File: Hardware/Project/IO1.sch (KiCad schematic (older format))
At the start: 1 part, among them U8 8255

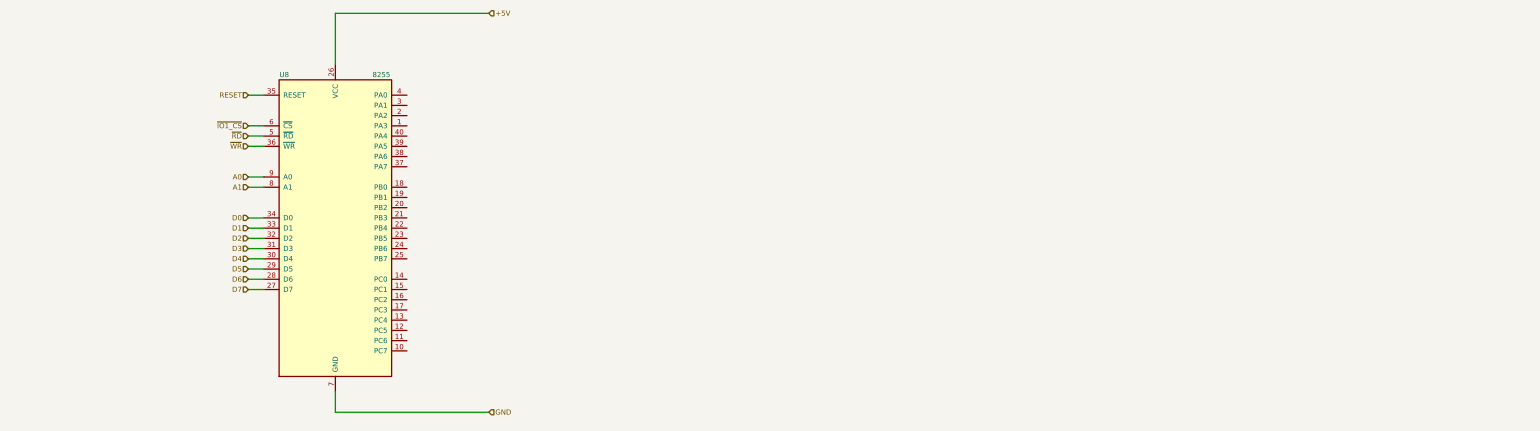
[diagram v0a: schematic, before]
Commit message: 1
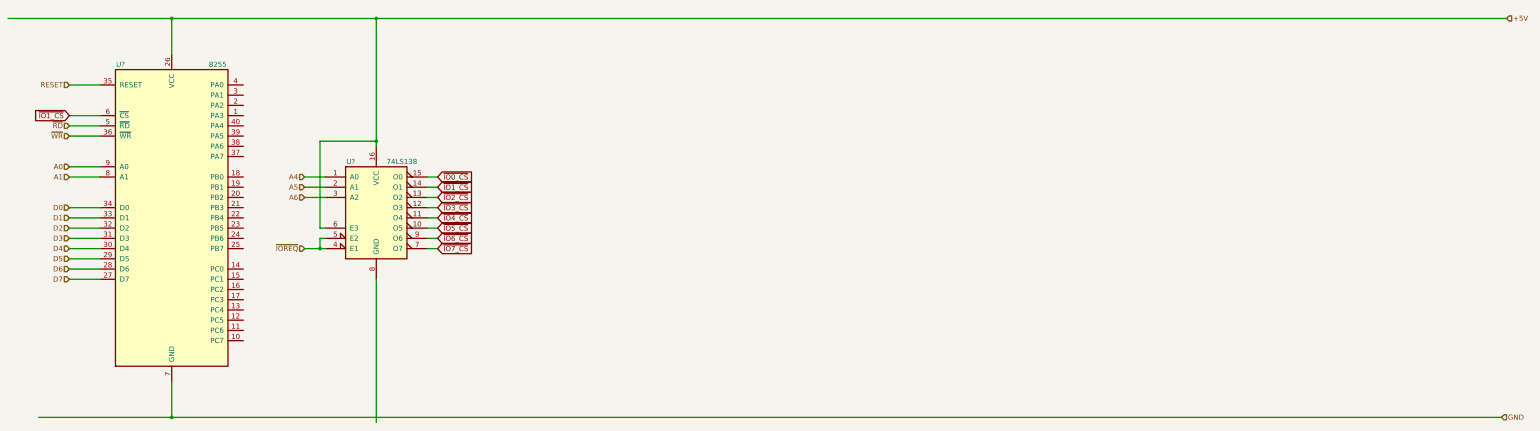
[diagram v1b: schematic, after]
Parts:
- removed U8: 8255, Package_DIP:DIP-40_W15.24mm, symbol Interface:8255
- added U?: 8255, Package_DIP:DIP-40_W15.24mm, symbol Interface:8255
- added U?: 74LS138, symbol 74xx:74LS138
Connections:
- net labels added: A4, A5, A6, ~IO0_CS, ~IO2_CS, ~IO3_CS, ~IO4_CS, ~IO5_CS, ~IO6_CS, ~IO7_CS, ~IOREQ
- wire segments 18 -> 42
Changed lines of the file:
@@
 EESchema Schematic File Version 4
+LIBS:8051-cache
 EELAYER 26 0
 EELAYER END
-$Descr A4 11693 8268
+$Descr A3 16535 11693
 encoding utf-8
-Sheet 4 5
+Sheet 5 6
 Title ""
 Date ""
@@
 Comment4 ""
 $EndDescr
-Text HLabel 3250 3500 0    50   Input ~ 0
+Text HLabel 15500 4750 2    50   Input ~ 0
+GND
+Text HLabel 15550 850  2    50   Input ~ 0
++5V
+$Comp
+L Interface:8255 U?
+U 1 1 5D59FA94
+P 2500 2800
+AR Path="/5DED3C2A/5D59FA94" Ref="U?"  Part="1"
+AR Path="/5DFCE73E/5D59FA94" Ref="U?"  Part="1"
+AR Path="/5E02D9A0/5D59FA94" Ref="U?"  Part="1"
+AR Path="/5D59EC5C/5D59FA94" Ref="U?"  Part="1"
+F 0 "U?" H 2000 4300 50  0000 C CNN
+F 1 "8255" H 2950 4300 50  0000 C CNN
+F 2 "Package_DIP:DIP-40_W15.24mm" H 2500 3100 50  0001 C CNN
+F 3 "http://aturing.umcs.maine.edu/~meadow/courses/cos335/Intel8255A.pdf" H 2500 3100 50  0001 C CNN
+	1    2500 2800
+	1    0    0    -1
+$EndComp
+Text HLabel 1500 3400 0    50   Input ~ 0
 D7
-Text HLabel 3250 3400 0    50   Input ~ 0
+Text HLabel 1500 3300 0    50   Input ~ 0
 D6
-Text HLabel 3250 3300 0    50   Input ~ 0
+Text HLabel 1500 3200 0    50   Input ~ 0
 D5
-Text HLabel 3250 3200 0    50   Input ~ 0
+Text HLabel 1500 3100 0    50   Input ~ 0
 D4
-Text HLabel 3250 3100 0    50   Input ~ 0
+Text HLabel 1500 3000 0    50   Input ~ 0
 D3
-Text HLabel 3250 3000 0    50   Input ~ 0
+Text HLabel 1500 2900 0    50   Input ~ 0
 D2
-Text HLabel 3250 2900 0    50   Input ~ 0
+Text HLabel 1500 2800 0    50   Input ~ 0
 D1
-Text HLabel 3250 2800 0    50   Input ~ 0
+Text HLabel 1500 2700 0    50   Input ~ 0
 D0
-Text HLabel 5600 4700 2    50   Input ~ 0
-GND
-Text HLabel 5600 800  2    50   Input ~ 0
-+5V
-Text HLabel 3250 2000 0    50   Input ~ 0
+Wire Wire Line
+	1800 2700 1500 2700
+Wire Wire Line
+	1800 2800 1500 2800
+Wire Wire Line
+	1800 2900 1500 2900
+Wire Wire Line
+	1800 3000 1500 3000
+Wire Wire Line
+	1800 3100 1500 3100
+Wire Wire Line
+	1800 3200 1500 3200
+Wire Wire Line
+	1800 3300 1500 3300
+Wire Wire Line
+	1800 3400 1500 3400
+Text HLabel 1500 2400 0    50   Input ~ 0
+A1
+Text HLabel 1500 2300 0    50   Input ~ 0
+A0
+Wire Wire Line
+	1800 2300 1500 2300
+Wire Wire Line
+	1800 2400 1500 2400
+Text HLabel 1500 2000 0    50   Input ~ 0
+~WR
+Text HLabel 1500 1900 0    50   Input ~ 0
 ~RD
-Text HLabel 3250 2100 0    50   Input ~ 0
-~WR
-Text HLabel 3250 1600 0    50   Input ~ 0
+Wire Wire Line
+	1800 1900 1500 1900
+Wire Wire Line
+	1800 2000 1500 2000
+Wire Wire Line
+	1800 1800 1500 1800
+Wire Wire Line
+	900  850  2500 850
+Wire Wire Line
+	1200 4750 2500 4750
+Wire Wire Line
+	2500 1200 2500 850
+Connection ~ 2500 850
+Wire Wire Line
+	2500 850  4500 850
+Wire Wire Line
+	2500 4400 2500 4750
+Connection ~ 2500 4750
+Wire Wire Line
+	2500 4750 15500 4750
+Text HLabel 1500 1500 0    50   Input ~ 0
 RESET
-Text HLabel 3250 2500 0    50   Input ~ 0
-A1
-Text HLabel 3250 2400 0    50   Input ~ 0
-A0
+Wire Wire Line
+	1800 1500 1500 1500
 $Comp
-L Interface:8255 U8
-U 1 1 5C8F2B3E
-P 4100 2900
-AR Path="/5E02D9A0/5C8F2B3E" Ref="U8"  Part="1"
-AR Path="/5E17A1DA/5C8F2B3E" Ref="U?"  Part="1"
-F 0 "U8" H 3600 4400 50  0000 C CNN
-F 1 "8255" H 4550 4400 50  0000 C CNN
-F 2 "Package_DIP:DIP-40_W15.24mm" H 4100 3200 50  0001 C CNN
-F 3 "http://aturing.umcs.maine.edu/~meadow/courses/cos335/Intel8255A.pdf" H 4100 3200 50  0001 C CNN
-	1    4100 2900
+L 74xx:74LS138 U?
+U 1 1 5D59FABE
+P 4500 2700
+AR Path="/5C68B4BB/5D59FABE" Ref="U?"  Part="1"
+AR Path="/5DED3C2A/5D59FABE" Ref="U?"  Part="1"
+AR Path="/5D59EC5C/5D59FABE" Ref="U?"  Part="1"
+F 0 "U?" H 4250 3150 50  0000 C CNN
+F 1 "74LS138" H 4750 3150 50  0000 C CNN
+F 2 "" H 4500 2700 50  0001 C CNN
+F 3 "http://www.ti.com/lit/gpn/sn74LS138" H 4500 2700 50  0001 C CNN
+	1    4500 2700
 	1    0    0    -1
 $EndComp
 Wire Wire Line
-	5600 800  4100 800
+	4500 2100 4500 2050
 Wire Wire Line
-	4100 800  4100 1300
+	4500 3400 4500 4800
+Text HLabel 3800 2600 0    50   Input ~ 0
+A6
+Text HLabel 3800 2500 0    50   Input ~ 0
+A5
+Text HLabel 3800 2400 0    50   Input ~ 0
+A4
 Wire Wire Line
-	5600 4700 4100 4700
+	4000 2400 3800 2400
 Wire Wire Line
-	4100 4700 4100 4500
+	4000 2500 3800 2500
 Wire Wire Line
-	3250 2800 3400 2800
+	4000 2600 3800 2600
 Wire Wire Line
-	3400 2900 3250 2900
+	4000 3000 3950 3000
 Wire Wire Line
-	3250 3000 3400 3000
+	3950 3000 3950 3100
 Wire Wire Line
-	3400 3100 3250 3100
+	3950 3100 4000 3100
 Wire Wire Line
-	3250 3200 3400 3200
+	4000 2900 3950 2900
 Wire Wire Line
-	3400 3300 3250 3300
+	3950 2900 3950 2050
 Wire Wire Line
-	3250 3400 3400 3400
+	3950 2050 4500 2050
+Connection ~ 4500 2050
 Wire Wire Line
-	3400 3500 3250 3500
+	4500 2050 4500 850
+Text GLabel 5100 2400 2    50   Input ~ 0
+~IO0_CS
+Connection ~ 3950 3100
 Wire Wire Line
-	3250 2000 3400 2000
+	5100 2400 5000 2400
+Text HLabel 3800 3100 0    50   Input ~ 0
+~IOREQ
 Wire Wire Line
-	3400 2100 3250 2100
-Wire Wire Line
-	3250 2400 3400 2400
-Wire Wire Line
-	3400 2500 3250 2500
-Wire Wire Line
-	3400 1600 3250 1600
-Text HLabel 3250 1900 0    50   Input ~ 0
+	3800 3100 3950 3100
+Text GLabel 5100 2500 2    50   Input ~ 0
 ~IO1_CS
 Wire Wire Line
-	3400 1900 3250 1900
+	5100 2500 5000 2500
+Text GLabel 5100 2600 2    50   Input ~ 0
+~IO2_CS
+Wire Wire Line
+	5100 2600 5000 2600
+Text GLabel 5100 2700 2    50   Input ~ 0
+~IO3_CS
+Wire Wire Line
+	5100 2700 5000 2700
+Text GLabel 5100 2800 2    50   Input ~ 0
+~IO4_CS
+Wire Wire Line
+	5100 2800 5000 2800
+Text GLabel 5100 2900 2    50   Input ~ 0
+~IO5_CS
+Wire Wire Line
+	5100 2900 5000 2900
+Text GLabel 5100 3000 2    50   Input ~ 0
+~IO6_CS
+Wire Wire Line
+	5100 3000 5000 3000
+Text GLabel 5100 3100 2    50   Input ~ 0
+~IO7_CS
+Wire Wire Line
+	5100 3100 5000 3100
+Text GLabel 1500 1800 0    50   Input ~ 0
+~IO1_CS
+Connection ~ 4500 850
+Wire Wire Line
+	4500 850  15550 850
 $EndSCHEMATC
